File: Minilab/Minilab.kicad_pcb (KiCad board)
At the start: 2 copper layers, 200 x 115 mm, 58 parts, among them J1 Salida, J2 Screw_Terminal_01x03, J3 Entradas, J4 Salidas, J5 Oscilador, J6 USB_C_Receptacle_USB2.0_14P, J7 DIN41612_02x16_AB, SW2 SW_DIP_x06, U1 4049, U2 NE555D, U78 LM7805_TO220

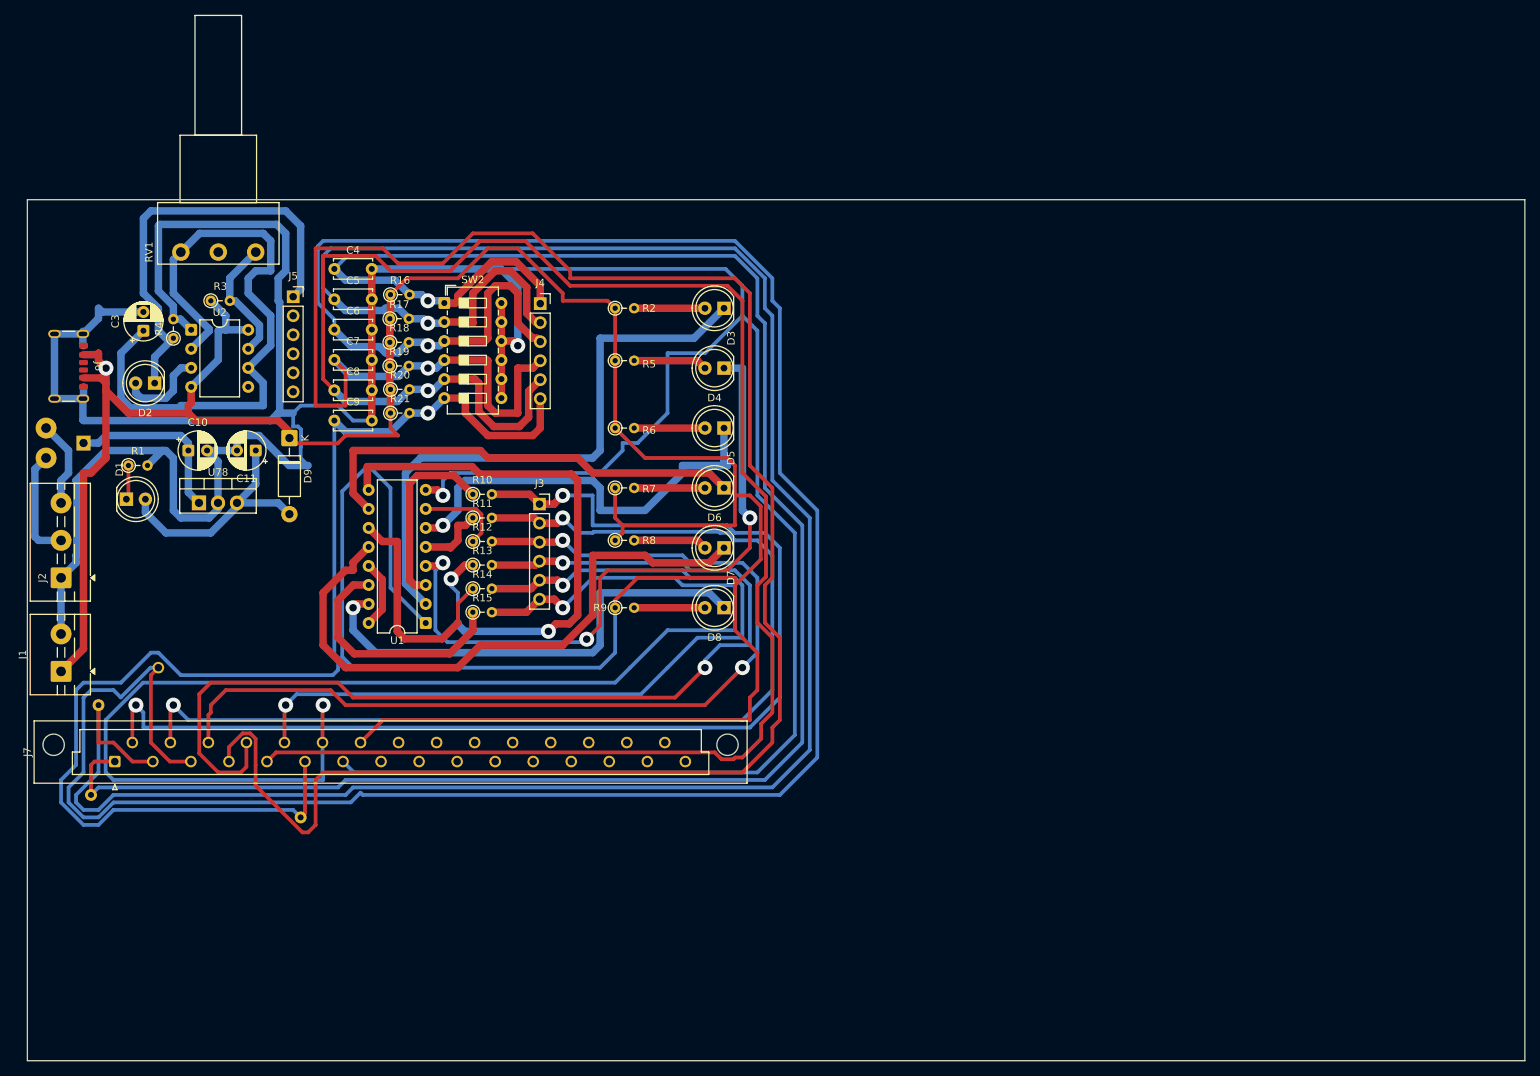
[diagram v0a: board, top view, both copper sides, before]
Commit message: Actualizacion3
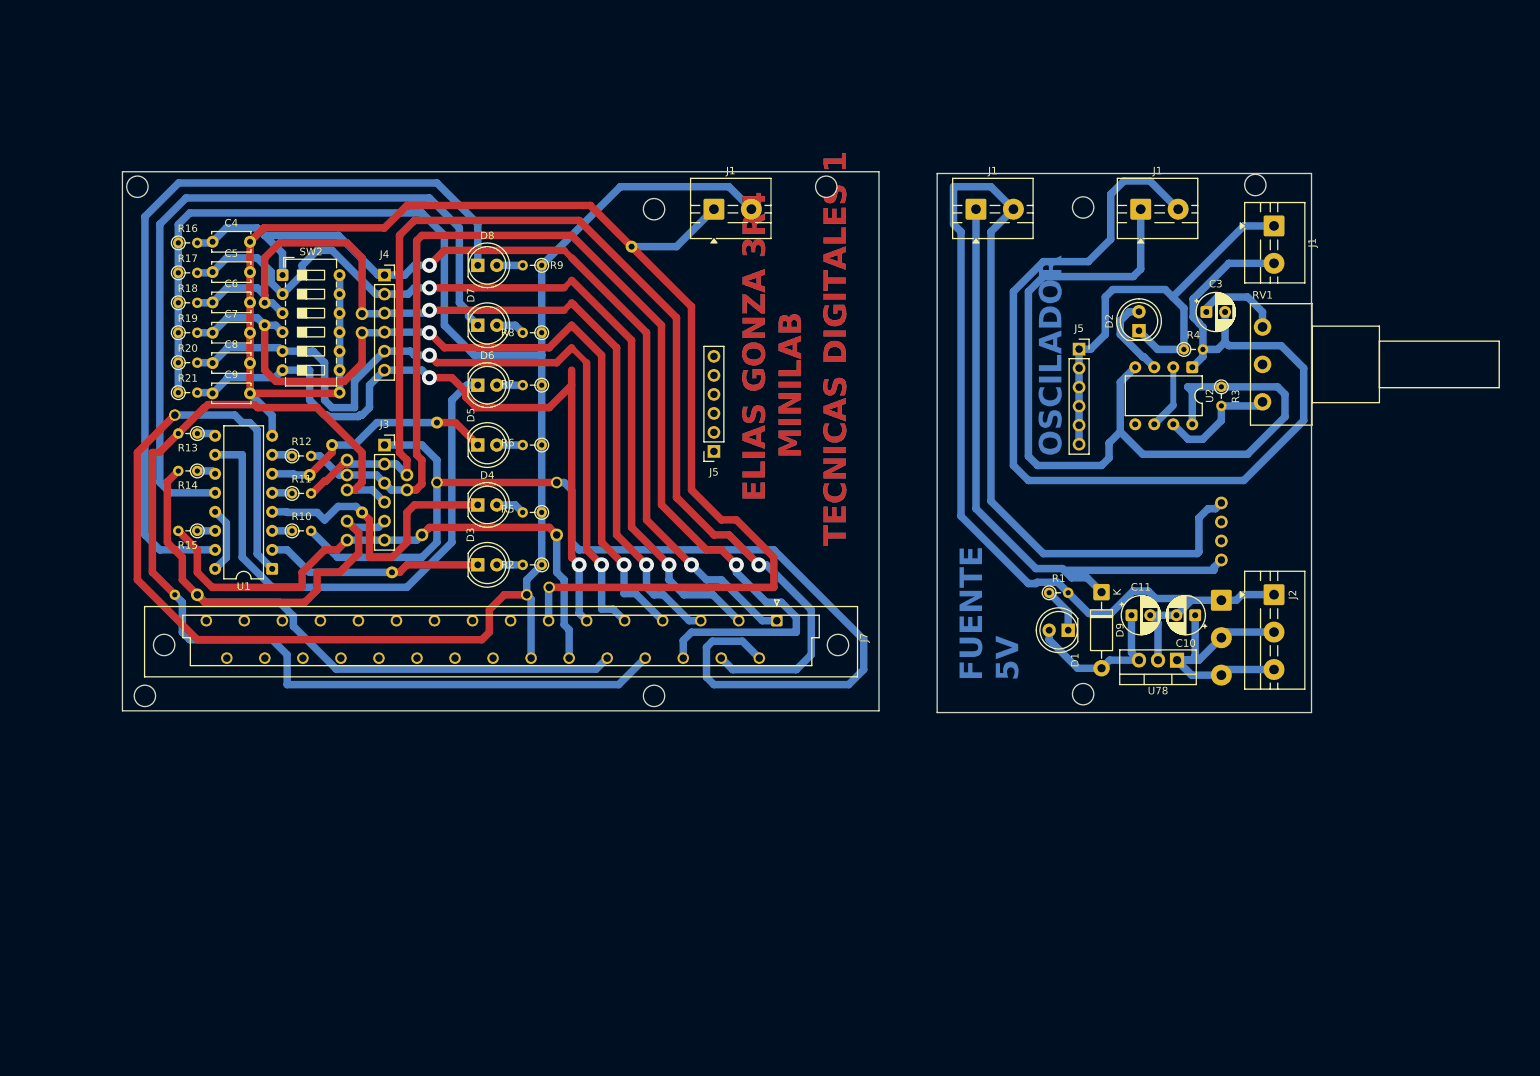
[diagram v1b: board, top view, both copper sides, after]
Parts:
- removed the ? at (31.0, 104.0)
- removed the ? at (59.0, 107.0)
- removed the ? at (32.0, 92.0)
- removed the ? at (30.0, 57.0)
- removed the ? at (25.0, 55.0)
- removed the ? at (25.0, 59.0)
- removed the ? at (40.0, 87.0)
- removed the J1 at (27.0, 87.5)
- removed the J5 at (58.0, 37.5)
- removed J6: USB_C_Receptacle_USB2.0_14P, Connector_USB:USB_C_Receptacle_GCT_USB4125-xx-x_6P_TopMnt_Horizontal
- added ?: , , F.Cu at (65.2, 59.3)
- added ?: , , F.Cu at (75.2, 69.3)
- added ?: , , F.Cu at (103.2, 30.8)
- added ?: , , F.Cu at (65.2, 63.3)
- added ?: , , F.Cu at (182.0, 65.0)
- added ?: , , F.Cu at (92.2, 76.3)
- added ?: , , F.Cu at (45.2, 77.3)
- added ?: , , F.Cu at (77.2, 54.3)
- added ?: , , F.Cu at (186.5, 22.5)
- added ?: , , F.Cu at (54.2, 38.3)
- added ?: , , F.Cu at (163.5, 25.5)
- added ?: , , F.Cu at (73.2, 63.3)
- added ?: , , F.Cu at (64.2, 50.3)
- added ?: , , F.Cu at (42.2, 77.3)
- added ?: , , F.Cu at (182.0, 83.0)
- added ?: , , F.Cu at (37.2, 22.8)
- added ?: , , F.Cu at (129.2, 22.8)
- added ?: , , F.Cu at (67.2, 39.7)
- added ?: , , F.Cu at (182.0, 78.0)
- added ?: , , F.Cu at (182.0, 67.5)
- added ?: , , F.Cu at (65.2, 67.4)
- added ?: , , F.Cu at (73.2, 61.3)
- added ?: , , F.Cu at (163.5, 90.5)
- added ?: , , F.Cu at (54.2, 41.3)
- added ?: , , F.Cu at (89.2, 77.3)
- added ?: , , F.Cu at (67.2, 42.3)
- added ?: , , F.Cu at (42.2, 53.3)
- added ?: , , F.Cu at (67.2, 66.3)
- added ?: , , F.Cu at (93.2, 62.3)
- added ?: , , F.Cu at (106.2, 90.8)
- added ?: , , F.Cu at (60.2, 61.3)
- added ?: , , F.Cu at (63.2, 57.3)
- added ?: , , F.Cu at (93.2, 69.3)
- added ?: , , F.Cu at (65.2, 70.0)
- added ?: , , F.Cu at (182.0, 88.0)
- added ?: , , F.Cu at (77.2, 62.3)
- added ?: , , F.Cu at (106.2, 25.8)
- added ?: , , F.Cu at (65.2, 61.3)
- added ?: , , F.Cu at (71.2, 74.3)
- added ?: , , F.Cu at (182.0, 70.1)
- added ?: , , F.Cu at (38.2, 90.8)
- added ?: , , F.Cu at (182.0, 72.6)
- added J1: Salida, TerminalBlock:TerminalBlock_MaiXu_MX126-5.0-02P_1x02_P5.00mm, F.Cu at (189.0, 28.0)
- added J1: Salida, TerminalBlock:TerminalBlock_MaiXu_MX126-5.0-02P_1x02_P5.00mm, F.Cu at (149.2, 25.8)
- added J1: Salida, TerminalBlock:TerminalBlock_MaiXu_MX126-5.0-02P_1x02_P5.00mm, F.Cu at (114.2, 25.8)
- added J1: Entrada, TerminalBlock:TerminalBlock_MaiXu_MX126-5.0-02P_1x02_P5.00mm, F.Cu at (171.2, 25.8)
- added J5: Oscilador, Connector_PinSocket_2.54mm:PinSocket_1x06_P2.54mm_Vertical, F.Cu at (114.2, 58.1)
- added J5: Oscilador, Connector_PinSocket_2.54mm:PinSocket_1x06_P2.54mm_Vertical, F.Cu at (163.0, 44.5)
- moved J2 162.0 mm to (189.0, 77.2), turned to -90 degrees
- moved C3 142.0 mm to (180.0, 39.5), turned to 0 degrees
- moved C10 136.3 mm to (178.5, 80.0), turned to 180 degrees
- moved RV1 135.9 mm to (187.5, 51.5), turned to 0 degrees
- moved R3 135.5 mm to (182.0, 49.5), turned to -90 degrees
- moved R4 135.0 mm to (177.0, 44.5), turned to 0 degrees
- moved U2 133.8 mm to (178.1, 46.9), turned to -90 degrees
- moved U78 132.3 mm to (176.0, 86.0), turned to 180 degrees
- moved D2 131.7 mm to (171.0, 42.0), turned to 90 degrees
- moved D1 127.0 mm to (161.5, 82.0), turned to 180 degrees
- moved R1 124.1 mm to (159.0, 77.0)
- moved C11 119.0 mm to (170.0, 80.0), turned to 0 degrees
- moved D9 110.4 mm to (166.0, 76.9)
- moved J7 95.2 mm to (125.1, 81.7), turned to -90 degrees
- moved D8 56.3 mm to (82.7, 33.3), turned to 0 degrees
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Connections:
- C10 pad 2: GND -> GND 1
- C11 pad 2: GND -> GND 1
- C3 pad 2: GND -> GND 2
- J2 pad 1: GND -> GND 1
- J7 pad b6: 5V -> E6
- R1 pad 2: GND -> GND 1
- R3 pad 1: 5V -> Net-(U2-VCC)
- R4 pad 2: GND -> GND 2
- U2 pad 1: GND -> GND 2
- U2 pad 4: 5V -> Net-(U2-VCC)
- U2 pad 8: 5V -> Net-(U2-VCC)
- U78 pad 2: GND -> GND 1
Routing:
- net GND: track 500.9 -> 212.2 mm, vias 2 -> 0
- net S3: track 331.9 -> 122.3 mm, vias 1 -> 2
- net GND 1: track 0.00 -> 195.2 mm
- net S2: track 301.6 -> 117.0 mm, vias 1 -> 2
- net S4: track 294.3 -> 113.3 mm, vias 1 -> 2
- net GND 2: track 0.00 -> 148.7 mm
- net S5: track 249.1 -> 104.1 mm, vias 1 -> 2
- net S1: track 264.0 -> 125.0 mm, vias 1 -> 2
- net Net-(U2-VCC): track 0.00 -> 118.5 mm
- net E6: track 177.2 -> 77.5 mm, vias 2 -> 0
- net Net-(R13-Pad1): track 77.7 -> 2.50 mm, vias 2 -> 0
- net S6: track 167.7 -> 98.7 mm, vias 1 -> 2
- net 5V: track 439.6 -> 371.7 mm, vias 1 -> 0
- net Net-(U2-THRES): track 87.6 -> 20.1 mm
- net Net-(D4-K): track 90.6 -> 39.6 mm, vias 3 -> 0
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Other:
- board size 200 x 115 mm -> 158.8 x 72.2 mm
- board text added: "ELIAS GONZA 3R4 MINILAB"
- board text added: "FUENTE 5V"
- board text added: "OSCILADOR"
- board text added: "TECNICAS DIGITALES 1"
